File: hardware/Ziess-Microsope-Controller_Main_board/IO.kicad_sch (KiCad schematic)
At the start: 27 parts, among them J16 Conn_01x10, J19 5787834-1, J20 031532951RFX, J21 Conn_01x10, U15 USBLC6-2SC6, U16 74LVC1G17, U19 ISO1430DWR

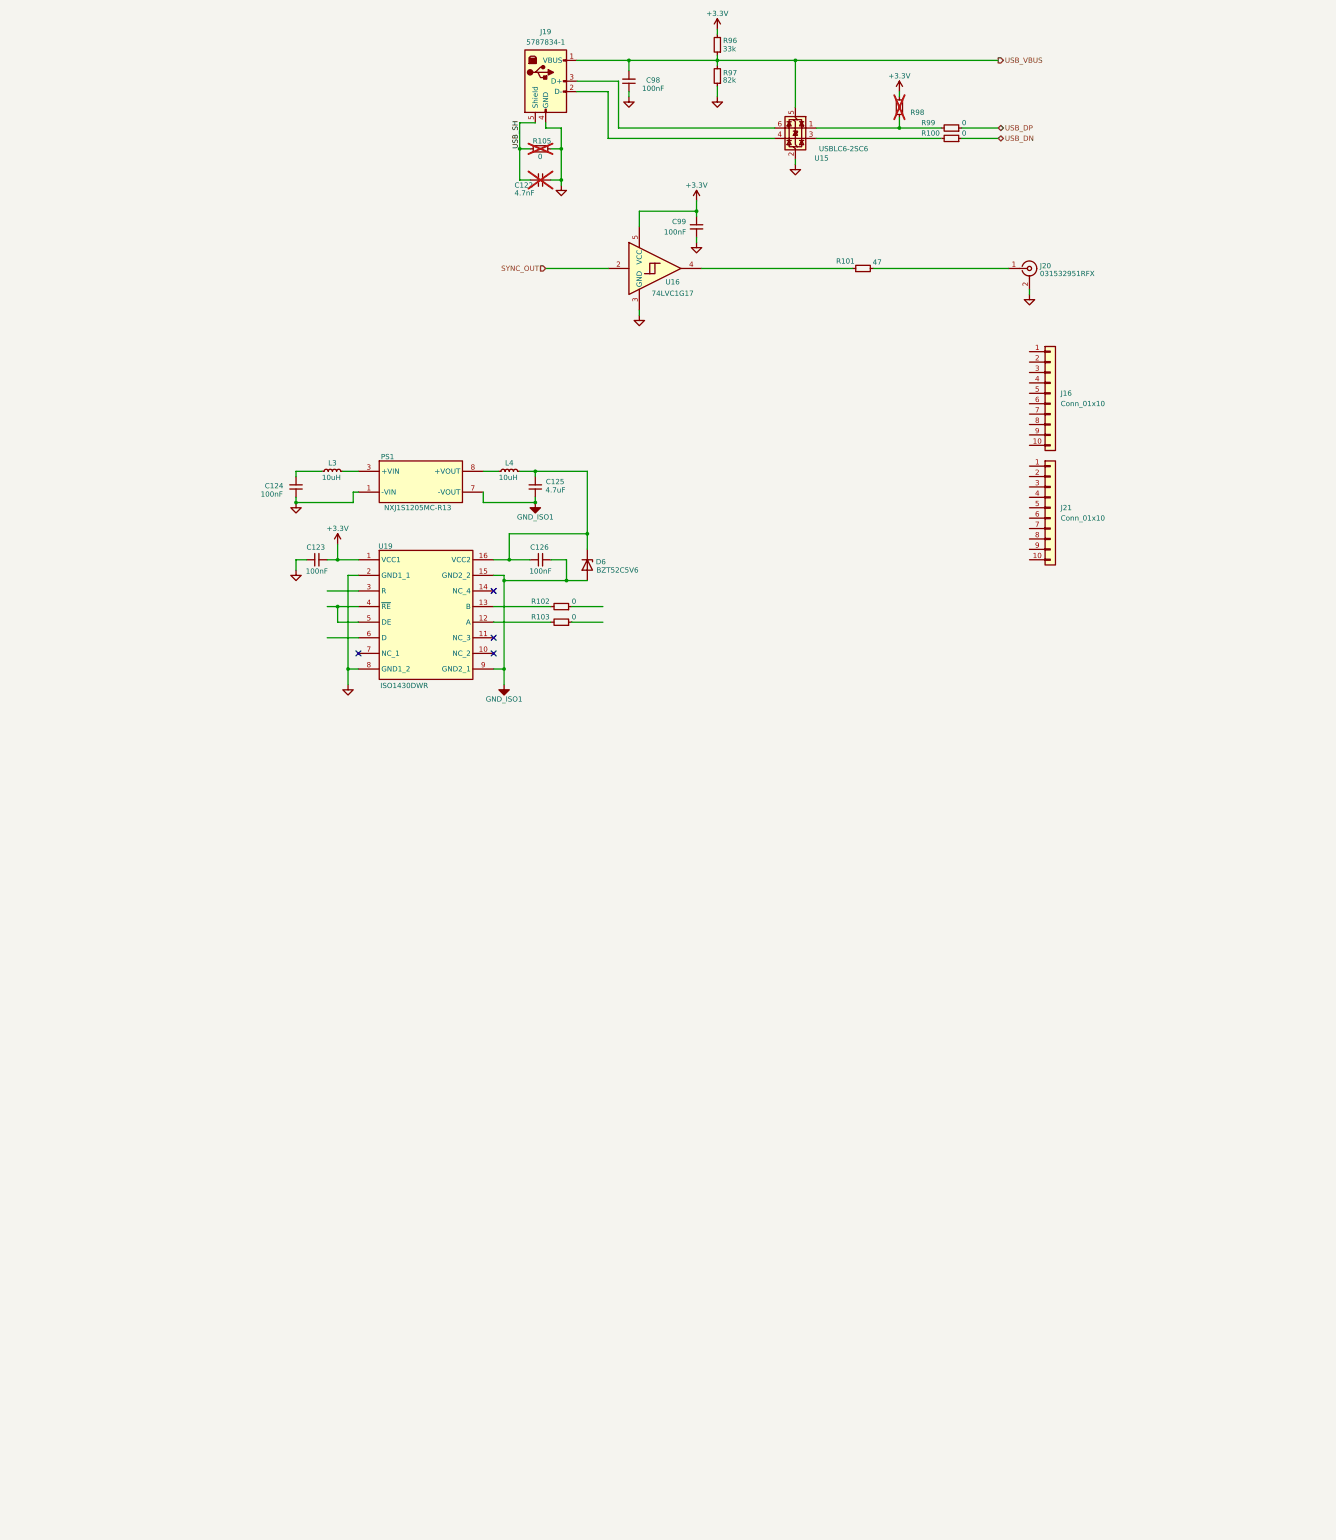
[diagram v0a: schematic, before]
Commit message: m
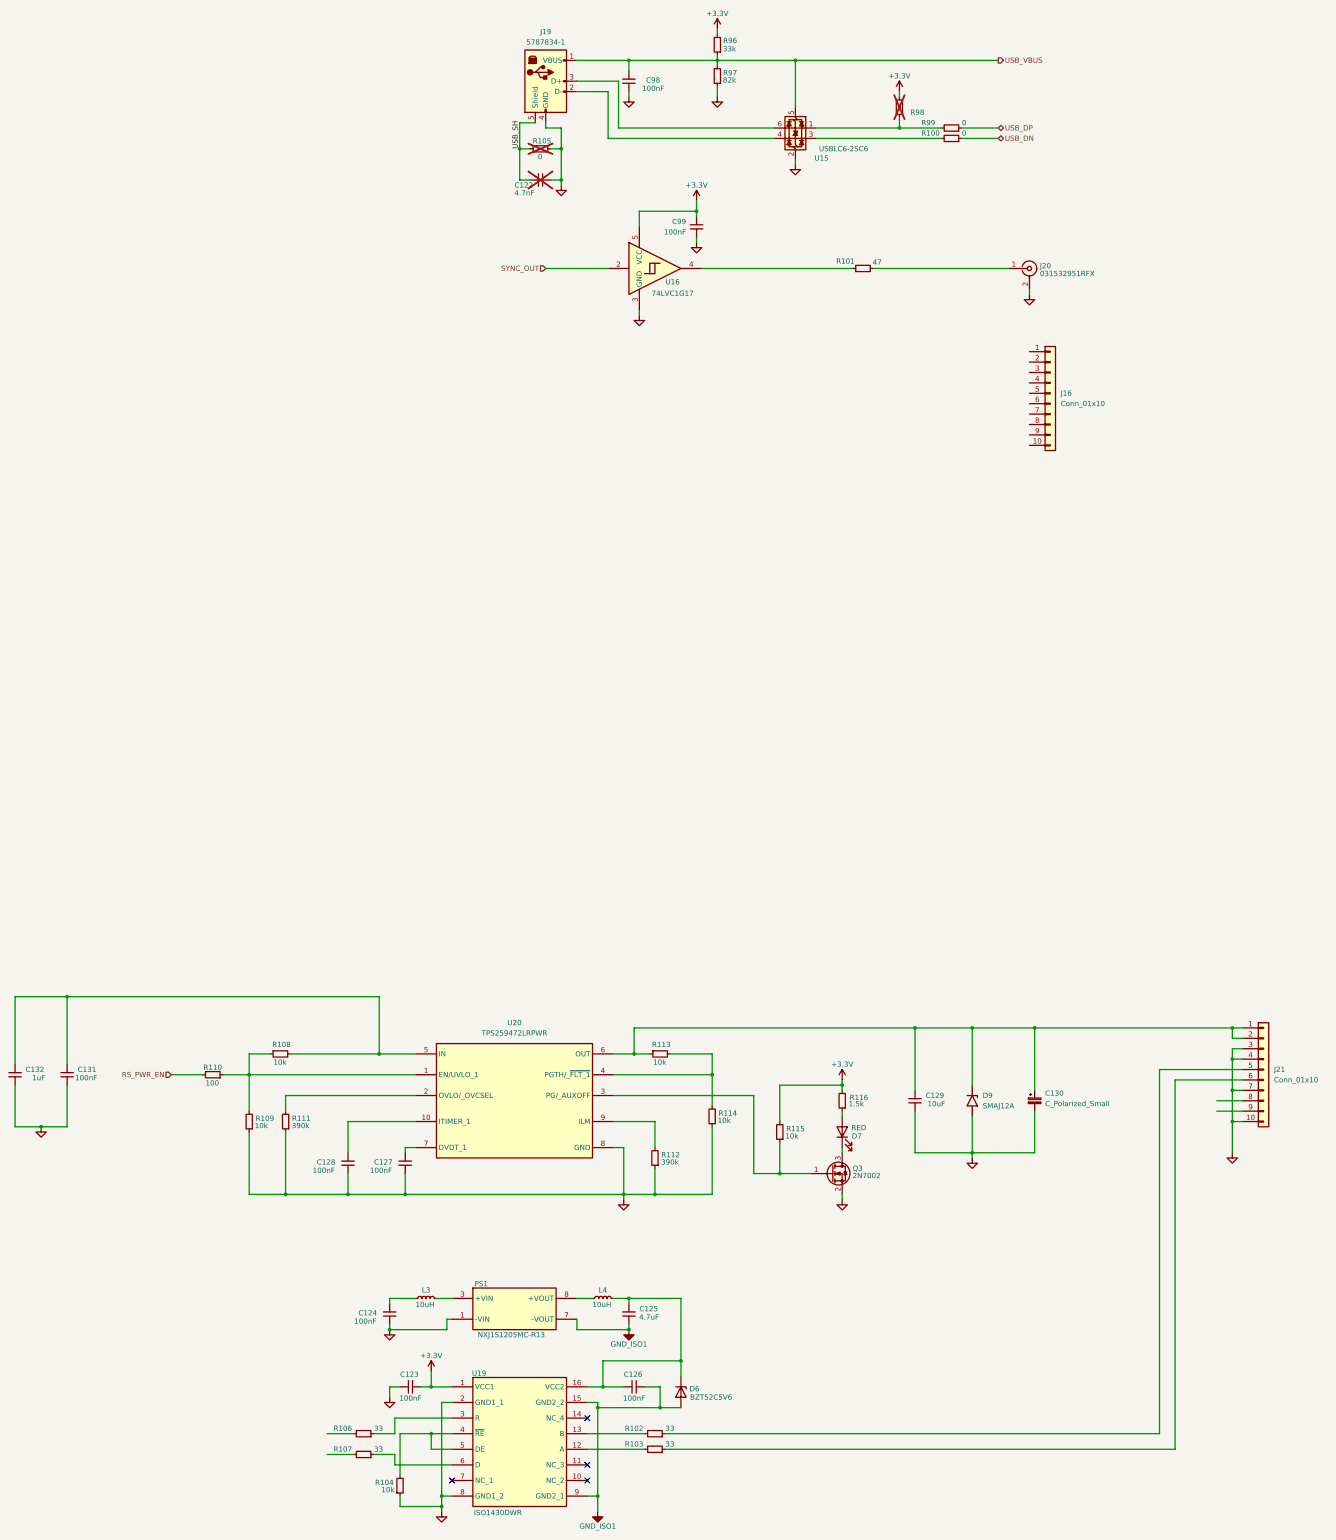
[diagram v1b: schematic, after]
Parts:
- added C127: 100nF, Capacitor_SMD:C_0402_1005Metric, symbol Device:C_Small
- added C128: 100nF, Capacitor_SMD:C_1206_3216Metric, symbol Device:C_Small
- added C129: 10uF, Capacitor_SMD:C_1206_3216Metric, symbol Device:C_Small
- added C130: C_Polarized_Small, Capacitor_SMD:CP_Elec_4x3, symbol Device:C_Polarized_Small
- added C131: 100nF, Capacitor_SMD:C_0603_1608Metric, symbol Device:C_Small
- added C132: 1uF, Capacitor_SMD:C_0603_1608Metric, symbol Device:C_Small
- added D7: RED, LED_SMD:LED_0603_1608Metric, symbol Device:LED
- added D9: SMAJ12A, Diode_SMD:D_SMC, symbol Diode:SMAJ12A
- added Q3: 2N7002, Package_TO_SOT_SMD:SOT-23, symbol Transistor_FET:2N7002
- added R104, R108, R109, R113, R114, R115: 10k, Resistor_SMD:R_0603_1608Metric, symbol Device:R_Small
- added R106, R107: 33, Resistor_SMD:R_0603_1608Metric, symbol Device:R_Small
- added R110: 100, Resistor_SMD:R_0603_1608Metric, symbol Device:R_Small
- added R111, R112: 390k, Resistor_SMD:R_0603_1608Metric, symbol Device:R_Small
- added R116: 1.5k, Resistor_SMD:R_0603_1608Metric, symbol Device:R_Small
- added U20: TPS259472LRPWR, Library:TPS259472LRPWR, symbol Library:TPS259472LRPWR
- C124: footprint Capacitor_SMD:C_0603_1608Metric -> Capacitor_SMD:C_1206_3216Metric
- C125: footprint Capacitor_SMD:C_0603_1608Metric -> Capacitor_SMD:C_0805_2012Metric
- J21: footprint (none) -> Library:BM10BGHSTBT
- R102, R103: value 0 -> 33
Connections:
- net +3.3V: now also R115.2, R116.2
- net GND: now also J21.10 (Pin_10), J21.3 (Pin_3), J21.4 (Pin_4), J21.7 (Pin_7), C127.1, C128.1, C129.1, C130.2, C131.1, C132.1, D9.2 (A2), Q3.2 (S), R104.1, R109.1, R111.1, R112.1, R114.1, U20.8 (GND)
- net at R103.1: now also J21.6 (Pin_6)
- net at J21.1 (Pin_1): now also J21.2 (Pin_2), C129.2, C130.1, D9.1 (A1), R113.1, U20.6 (OUT)
- net at J21.5 (Pin_5): now also R102.1
- net at U19.3 (R): now also R106.1
- net at U19.4 (~{RE}), U19.5 (DE): now also R104.2
- net at U19.6 (D): now also R107.1
- new net: C131.2, C132.2, R108.2, U20.5 (IN)
- new net: Q3.1 (G), R115.1, U20.3 (PG/_AUXOFF)
- new net: D7.1 (K), Q3.3 (D)
- new net: D7.2 (A), R116.1
- new net: R108.1, R109.2, R110.1, U20.1 (EN/UVLO_1), U20.11 (EN/UVLO_2)
- new net: C128.2, U20.10 (ITIMER_1), U20.14 (ITIMER_2)
- new net: R113.2, R114.2, U20.12 (PGTH/_~{FLT_2}), U20.4 (PGTH/_~{FLT_1})
- new net: C127.2, U20.13 (DVDT_2), U20.7 (DVDT_1)
- new net: R111.2, U20.2 (OVLO/_OVCSEL)
- new net: R112.2, U20.9 (ILM)
- new net RS_PWR_EN: R110.2
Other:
- moved on the sheet: C123, C124, C125, C126, D6, J21, L3, L4, PS1, R102, R103, U19
